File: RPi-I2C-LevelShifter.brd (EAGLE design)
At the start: 16.2 x 29.2 mm, 8 parts, among them Q1 2N7002, Q2 2N7002

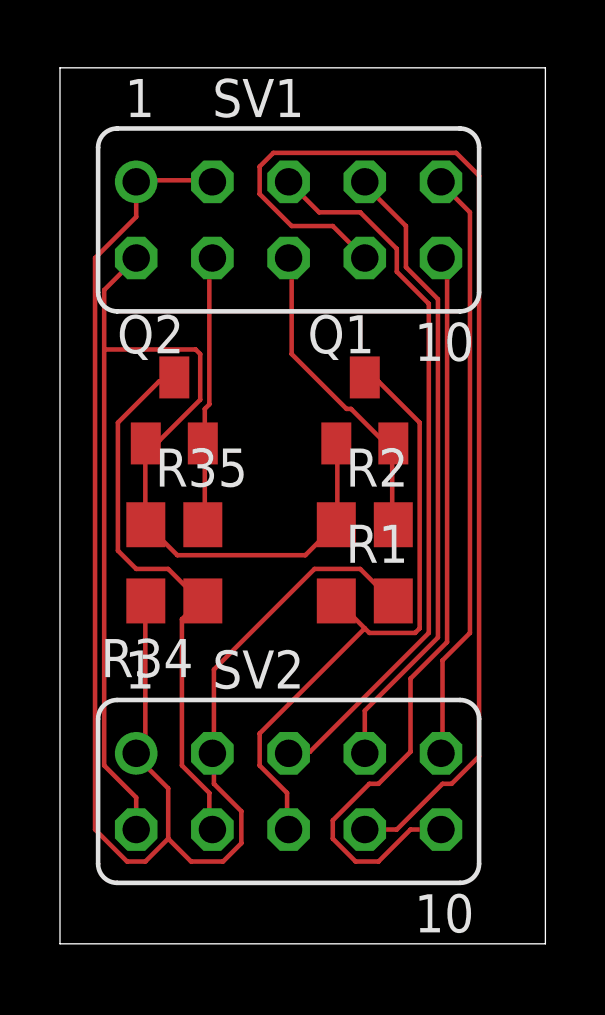
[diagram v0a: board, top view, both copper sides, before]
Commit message: added simulation; improved layout
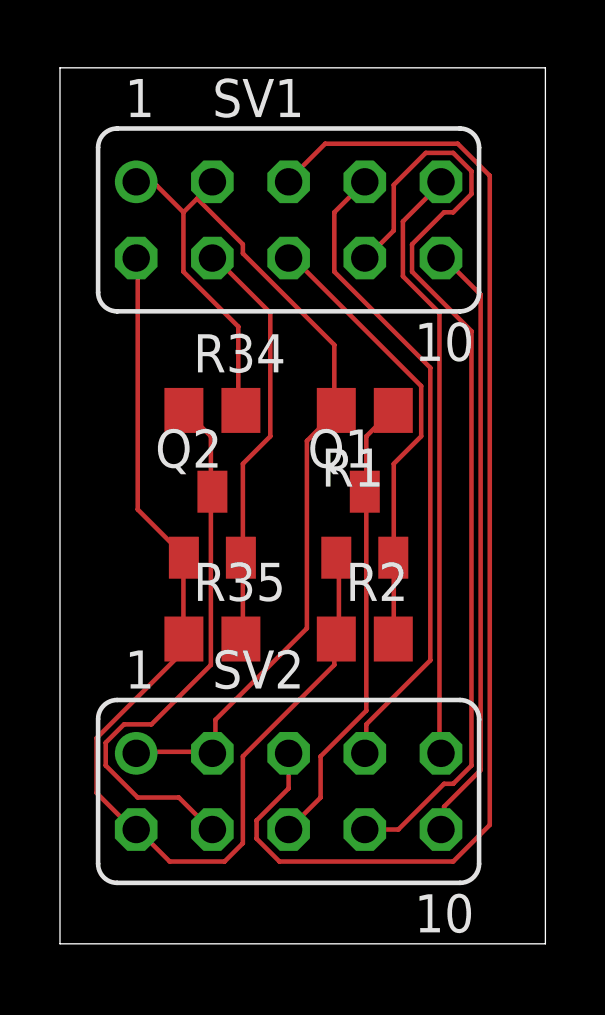
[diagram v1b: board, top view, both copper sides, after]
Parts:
- moved R34 6.48 mm to (5.08, 17.8), turned to 0 degrees
- moved R1 6.35 mm to (10.2, 17.8), turned to 180 degrees
- moved Q2 4.02 mm to (5.08, 14.0)
- moved R35 4.02 mm to (5.08, 10.2)
- moved Q1 3.81 mm to (10.2, 14.0)
- moved R2 3.81 mm to (10.2, 10.2)
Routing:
- net +5V: track 53.5 -> 35.6 mm
- net GND: track 24.1 -> 41.2 mm
- net SCL_OUT: track 21.3 -> 15.5 mm
- net P10: track 25.6 -> 20.3 mm
- net P8: track 37.3 -> 32.2 mm
- net SDA_IN: track 9.14 -> 14.0 mm
- net SCL_IN: track 10.7 -> 15.0 mm
- net +3V3: track 39.7 -> 36.7 mm
- net P7: track 21.1 -> 21.7 mm
